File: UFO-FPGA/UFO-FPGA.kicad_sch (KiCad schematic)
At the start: 0 parts

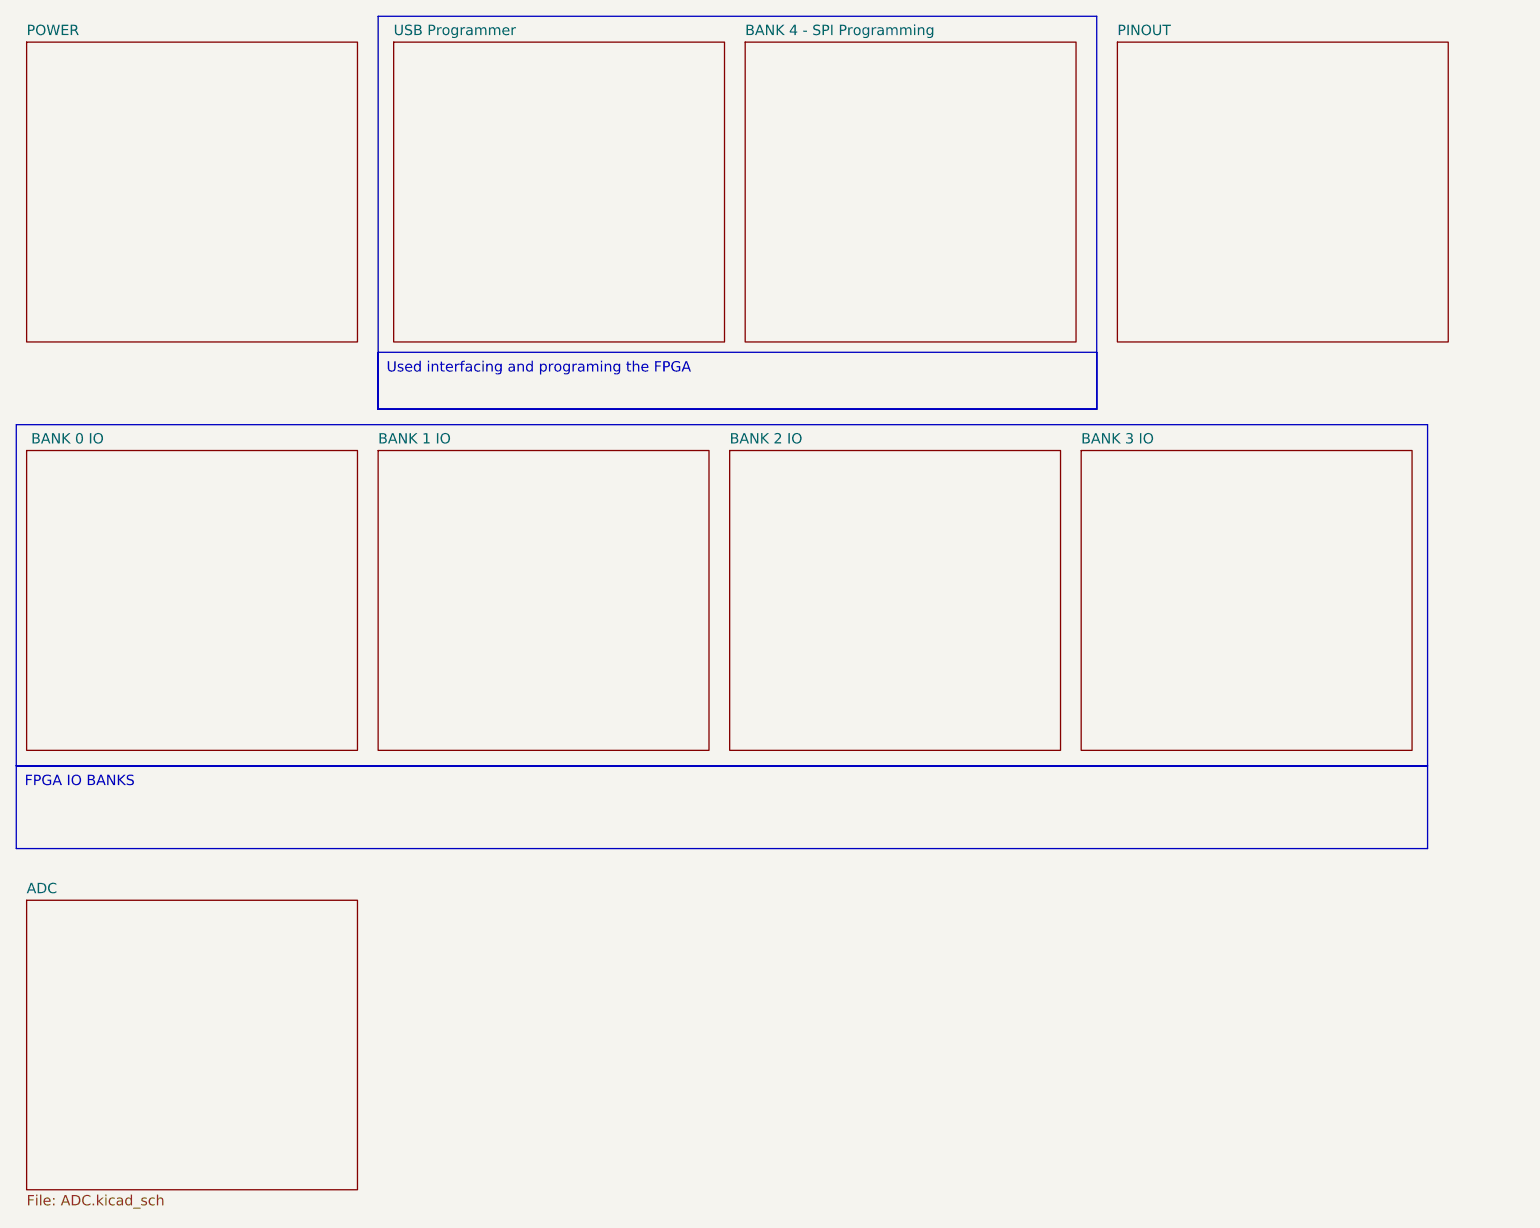
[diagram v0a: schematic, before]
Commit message: schema
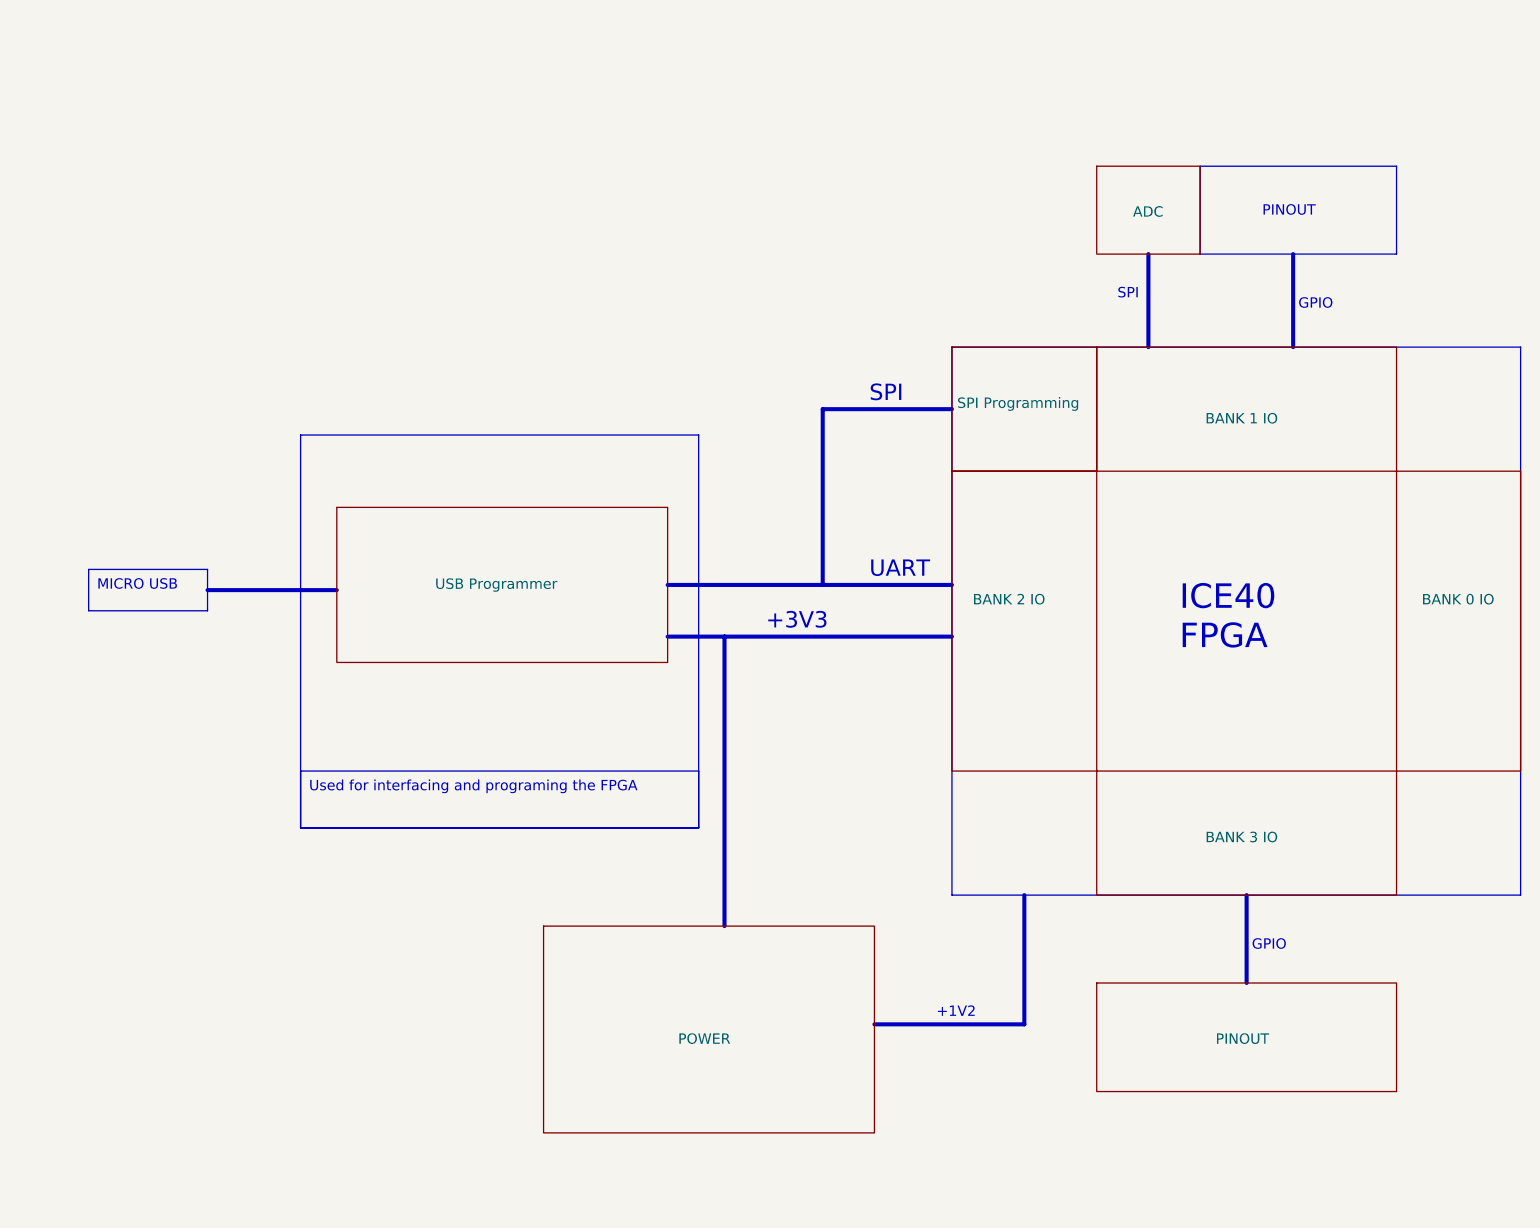
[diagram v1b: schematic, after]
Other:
- sheet BANK 4 - SPI Programming renamed SPI Programming
- note added: "+1V2"
- note added: "+3V3"
- note added: "GPIO"
- note added: "ICE40 FPGA"
- note added: "PINOUT"
- note added: "SPI"
- note added: "UART"
- title: (none) -> UFO-FPGA BLOCK diagram
